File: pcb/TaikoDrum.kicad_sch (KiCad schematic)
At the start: 26 parts, among them J1 USB_B_Micro, J2 Conn_02x04_Odd_Even, U1 STM32F103C8Tx, U2 LM3940IMPX-3.3_NOPB, Y1 8Mhz

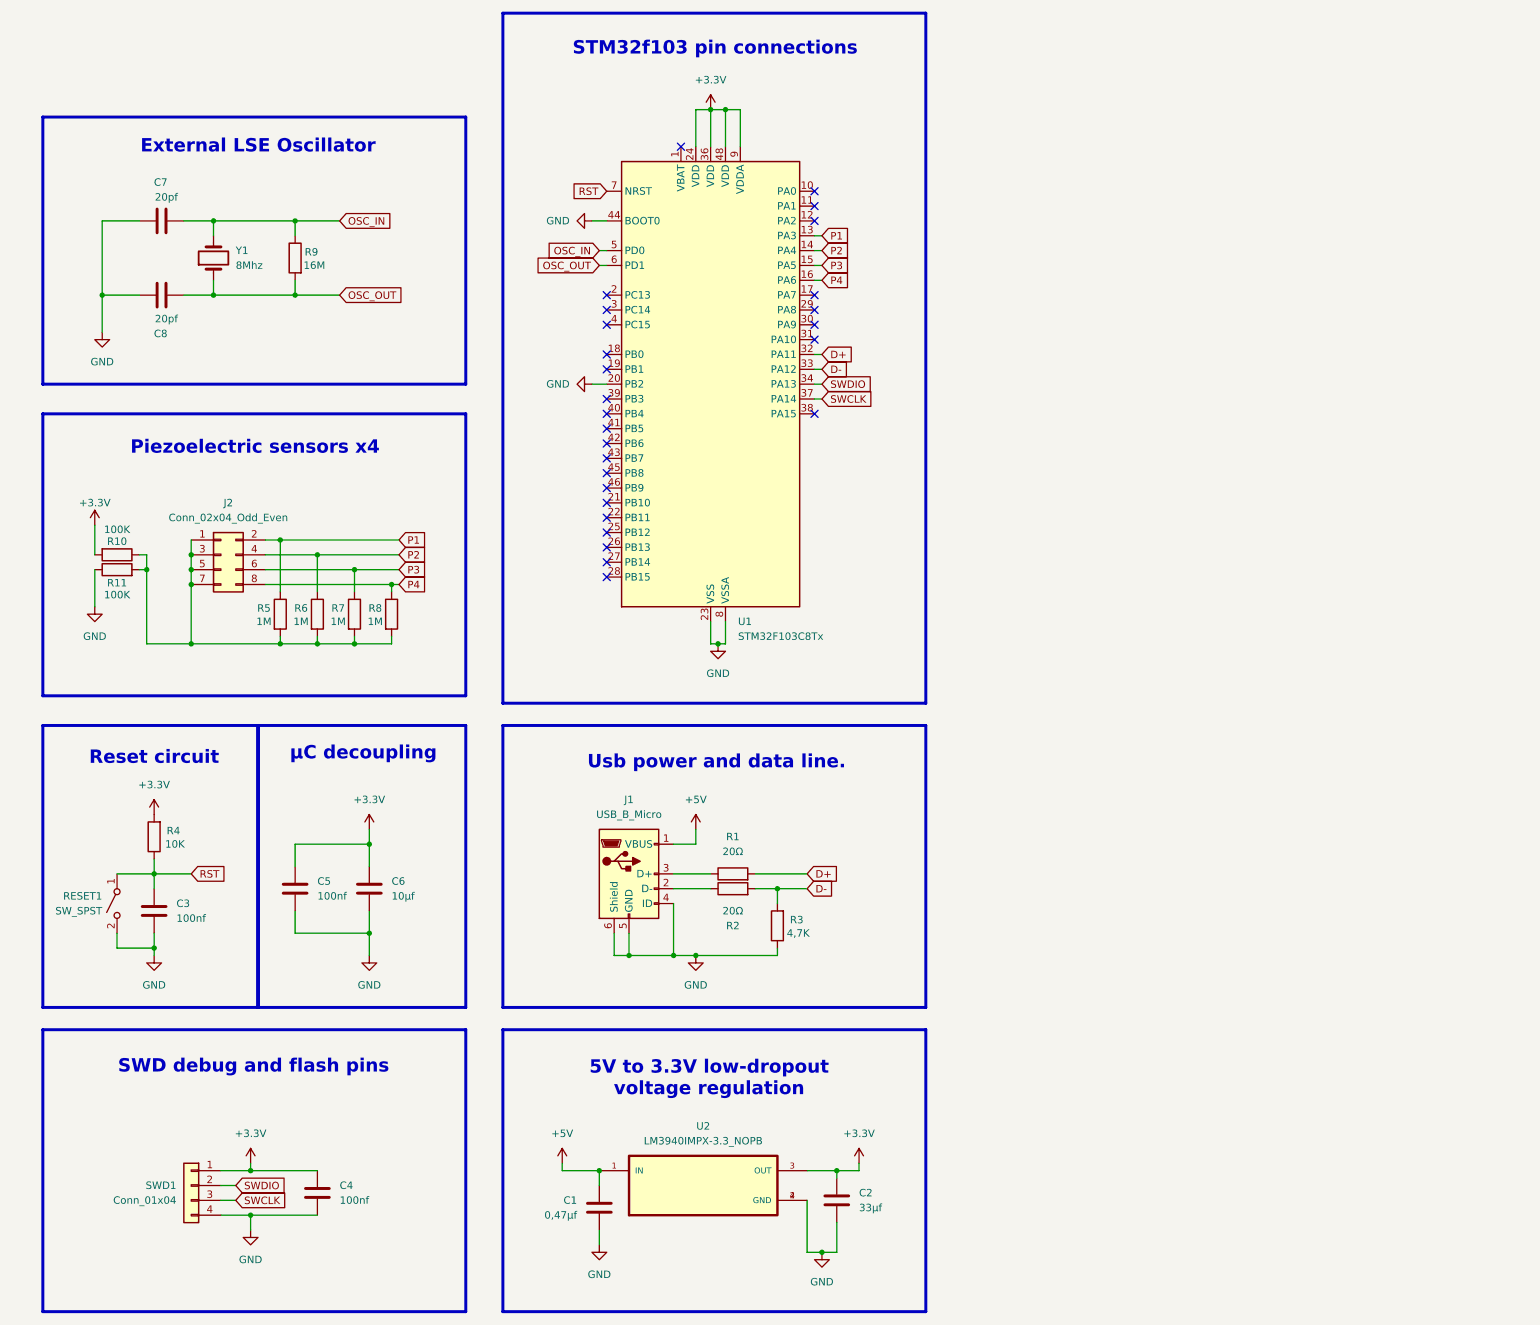
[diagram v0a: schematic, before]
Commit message: Updated PCB schematic.
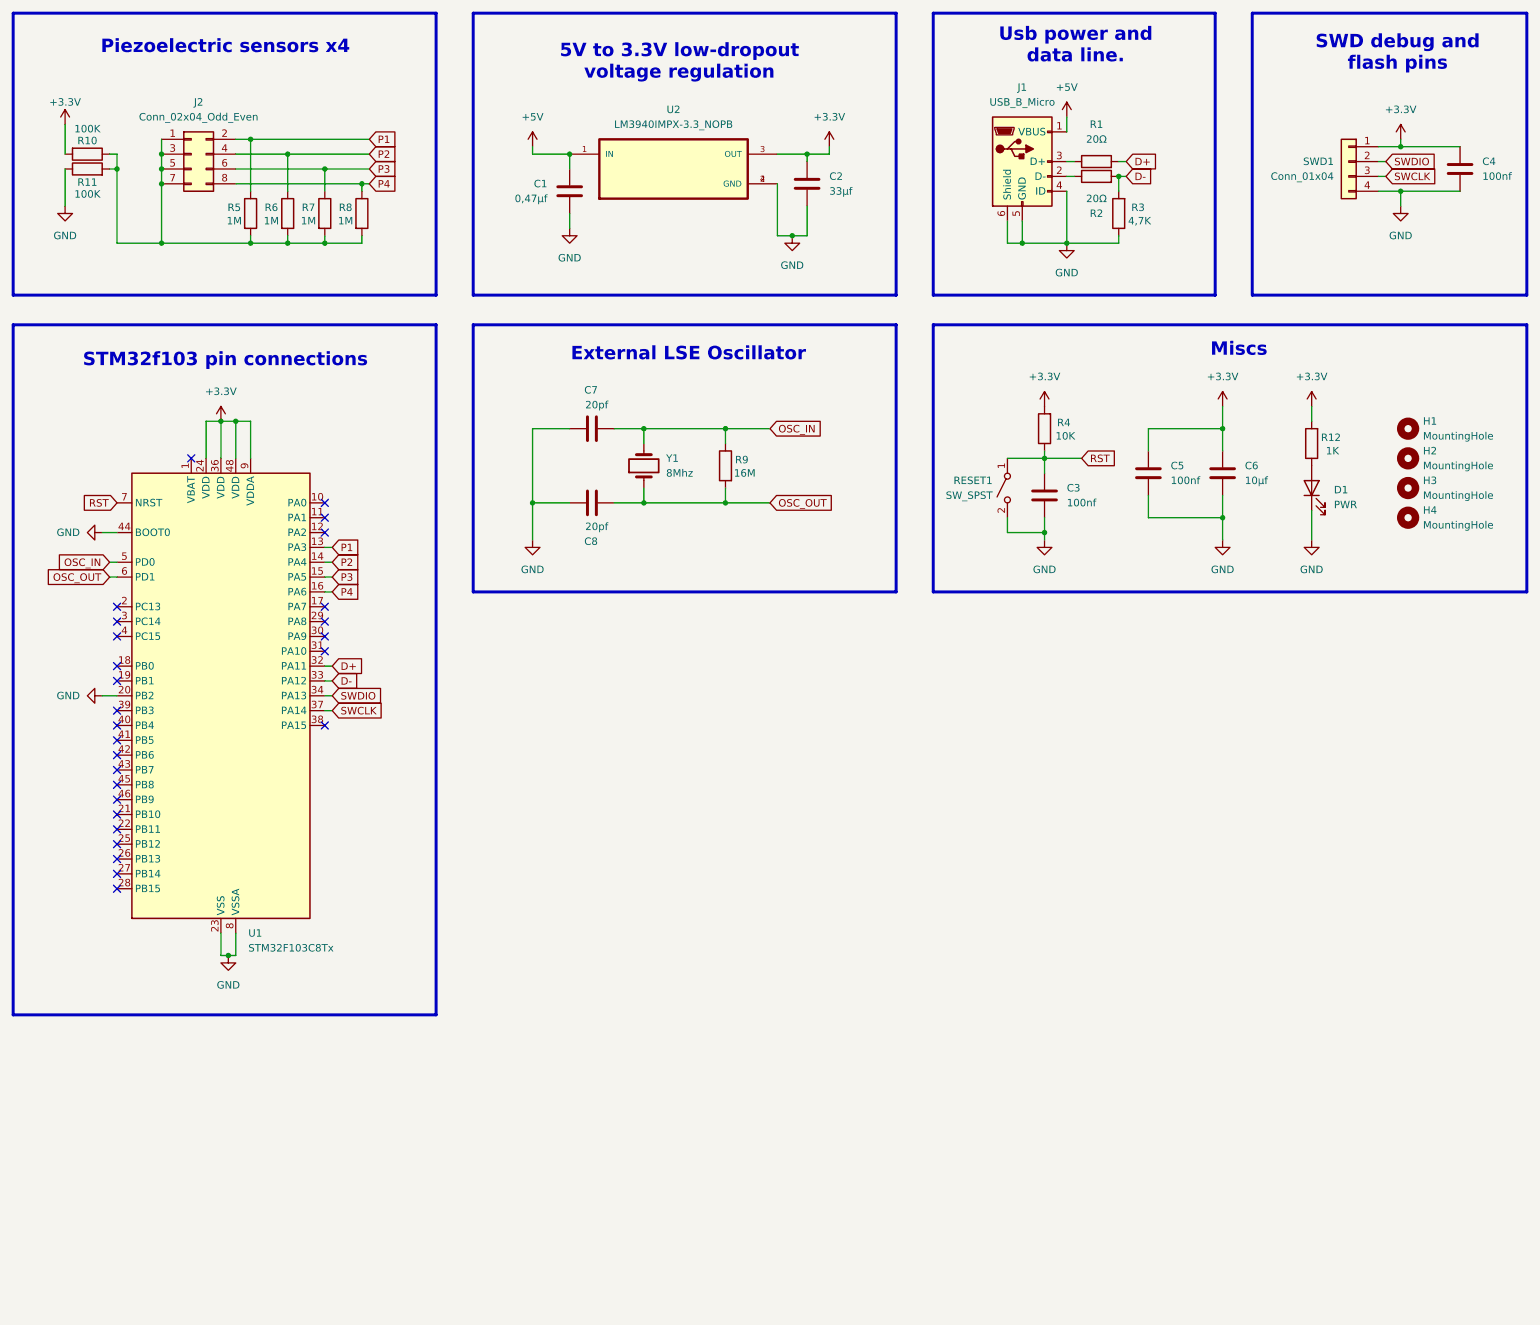
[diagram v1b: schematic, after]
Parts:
- added D1: PWR, LED_THT:LED_D3.0mm, symbol Device:LED
- added H1, H2, H3, H4: MountingHole, MountingHole:MountingHole_2.2mm_M2, symbol Mechanical:MountingHole
- added R12: 1K, Resistor_THT:R_Axial_DIN0204_L3.6mm_D1.6mm_P2.54mm_Vertical, symbol Device:R
- C3, C4, C5, C6, C7, C8: footprint Capacitor_SMD:C_0805_2012Metric_Pad1.18x1.45mm_HandSolder -> Capacitor_THT:C_Radial_D5.0mm_H5.0mm_P2.00mm
- R1, R10, R11, R2, R3, R4, R5, R6, R7, R8, R9: footprint Resistor_SMD:R_0805_2012Metric -> Resistor_THT:R_Axial_DIN0204_L3.6mm_D1.6mm_P2.54mm_Vertical
- Y1: footprint (none) -> Crystal:Crystal_HC52-U_Vertical
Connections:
- net +3.3V: now also R12.2
- net GND: now also D1.1 (K)
- new net: D1.2 (A), R12.1
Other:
- note added: "Miscs"
- note removed: "Reset circuit"
- note removed: "µC decoupling"
- moved on the sheet: C1, C2, C3, C4, C5, C6, C7, C8, J1, J2, R1, R10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
